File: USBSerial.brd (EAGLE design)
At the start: 45.8 x 26 mm, 28 parts, among them IC1 ATMEGA16U2, IC2 LD1117-33, J1 ISP, J2 USB, J5 DFU, J6 Serial, J8 Gnd, J9 VDD Select, Q1 16MHz

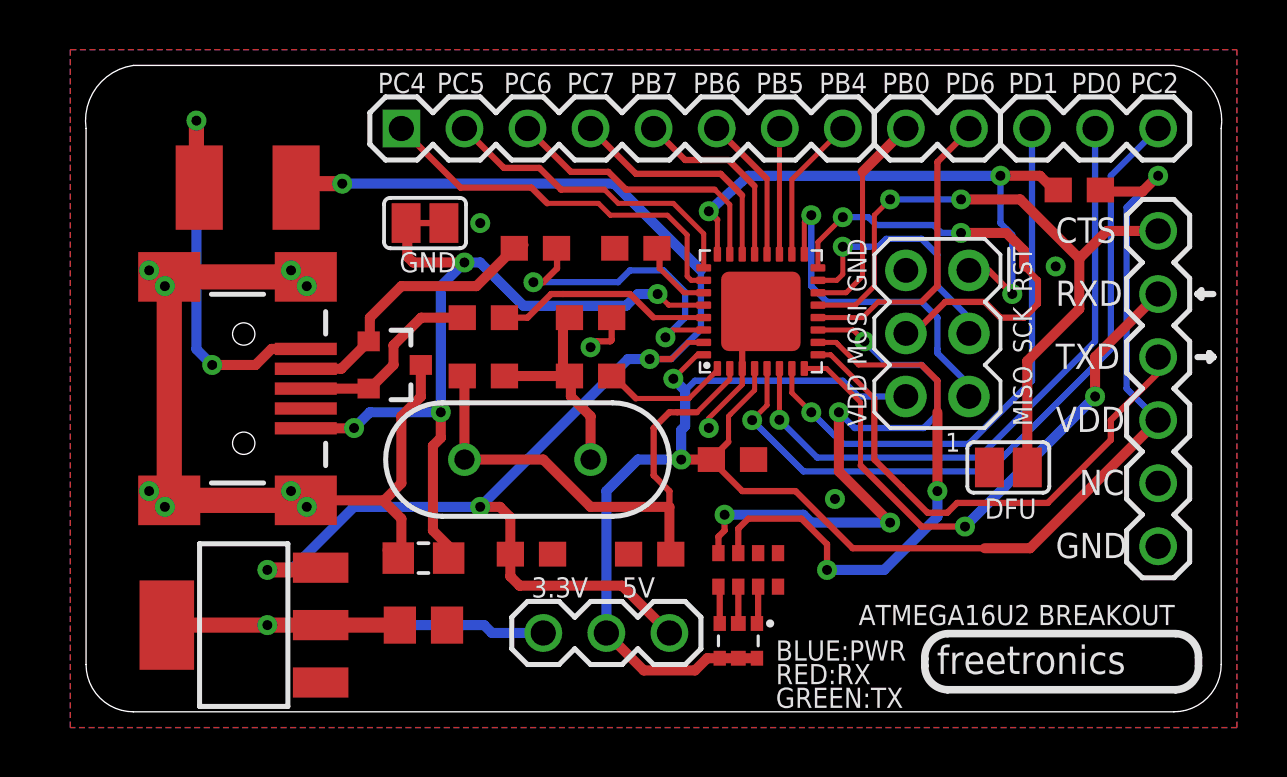
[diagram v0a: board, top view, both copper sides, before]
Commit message: Preparation for v1.0 release
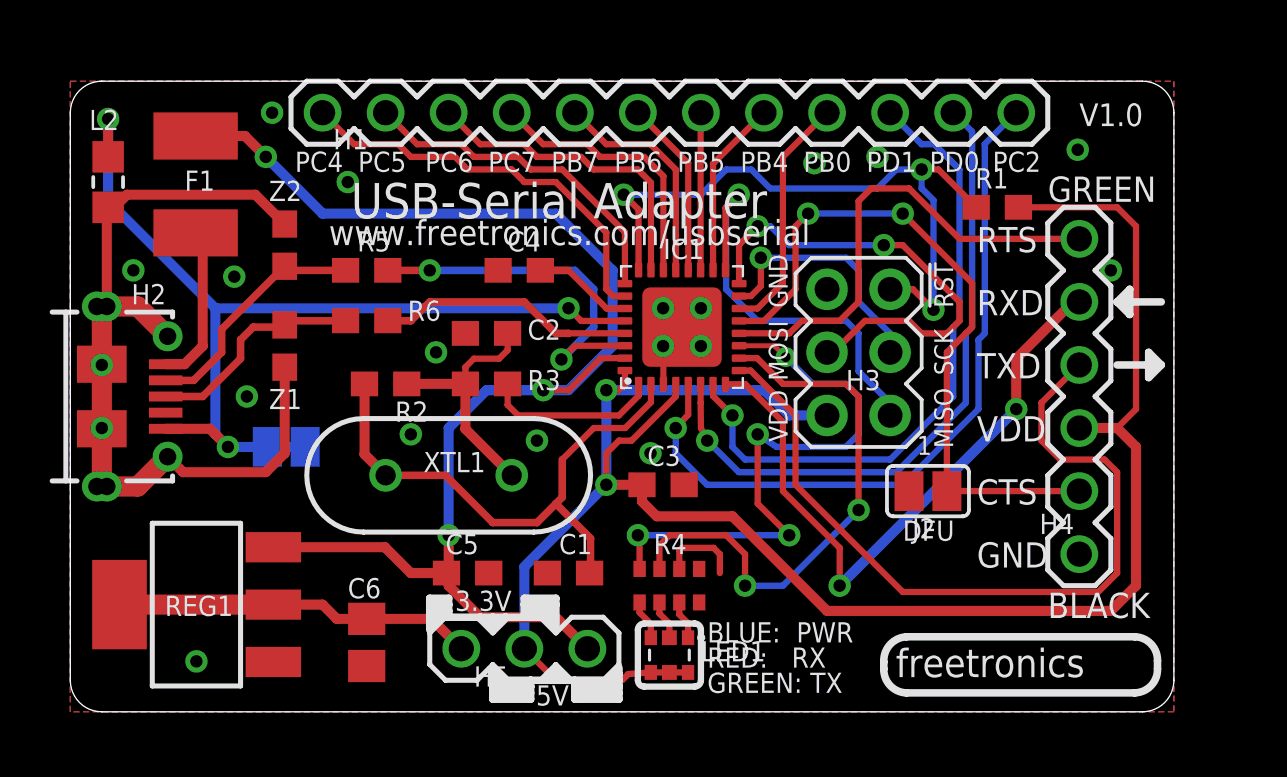
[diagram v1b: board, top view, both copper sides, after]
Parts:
- removed IC2: LD1117-33, freetronics-luke:SOT-223
- removed J3: (no value), freetronics-master-v1:1X02
- removed J4: (no value), freetronics-master-v1:1X08
- removed J5: DFU, freetronics-luke:SJ
- removed J6: Serial, freetronics-master-v1:1X06
- removed J7: (no value), freetronics-master-v1:1X03
- removed J8: Gnd, freetronics-luke:SJ
- removed J9: VDD Select, freetronics-luke:JUMPER_SPDT
- removed L1: Ferrite bead 0805, freetronics-master-v1:0805-LARGE
- removed Q1: 16MHz, freetronics-master-v1:HC49US
- added H1: M12PTH, freetronics-original:1X12
- added H2: USB-6PSMT, freetronics-jon:USB-MICROB-MB05PMXX
- added H3: ICSP, freetronics-luke:HEADER_2X3
- added H4: Serial, freetronics-master-v1:1X06
- added H5: VDD Select, freetronics-luke:JUMPER_SPDT
- added L2: 0805 INDUCTOR, freetronics-master-v1:0805-LARGE
- added REG1: LD1117-33 SOT-223, freetronics-luke:SOT-223
- added XTL1: 16MHz, freetronics-master-v1:HC49US
- added Z2: PGB1010603, freetronics:0603
- C1, C2: value 22p -> 22p 0603
- C3: value 100n -> 100n 0603
- C4: value 1uF -> 1uF 0603
- C5: value 10uF -> 100n 0603; device freetronics-jon:C0805 -> freetronics:0603
- C6: value 100n -> 10uF 10V ceramic 0805; device freetronics:0603 -> freetronics-jon:C0805
- F1: value 500mA PTC -> 500mA PTC 1812
- IC1: value ATMEGA16U2 -> ATMEGA16U2 QFN-32
- J1: value ISP -> Gnd; device freetronics-luke:HEADER_2X3 -> freetronics-jon:SJC
- J2: value USB -> DFU; device freetronics-luke:USB-MINIB-FT -> freetronics-luke:SJ
- R1: value 10k -> 10k 0603
- R2: value 1M -> 1M 0603
- R3: value 27R -> 27R 0603
- R5, R6: value 22R -> 22R 0603
- Z1: value PGB102ST23 -> PGB1010603; device freetronics-luke:SOT23-3 -> freetronics:0603
- moved J2 29.1 mm to (34.5, 8.89)
- moved J1 26.6 mm to (8.70, 10.7), flipped to the bottom, turned to 0 degrees
- moved C6 7.53 mm to (11.9, 2.79), turned to 270 degrees
- moved R5 6.85 mm to (11.9, 17.8)
- moved C4 4.78 mm to (18.1, 17.8)
- moved R6 4.70 mm to (11.9, 15.7)
- moved Z1 4.45 mm to (8.64, 14.7)
- moved C2 4.24 mm to (16.8, 15.2), turned to 0 degrees
- moved R3 4.20 mm to (16.8, 13.2)
- moved R2 3.95 mm to (12.7, 13.2)
- moved R1 3.38 mm to (37.3, 20.3)
- moved C1 3.36 mm to (20.1, 5.59)
- moved R4 3.24 mm to (24.1, 5.08)
- moved IC1 3.24 mm to (24.6, 15.5)
- moved C3 2.97 mm to (23.9, 9.14)
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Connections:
- removed net N$3: J2.SH1, J2.SH2, J2.SH3, J2.SH4, L1.1, Z1.3
- removed net PD6: IC1.12, J3.2
- new net N$8: H2.FIX1, H2.FIX2, H2.PIN1, H2.PIN2, H2.TAB1, H2.TAB2, L2.2, Z1.2, Z2.2
- new net RTS: H4.6, IC1.12
- net !RESET: now also H3.5; no longer J1.5
- net +3V3: now also C6.1, H5.1, REG1.2, REG1.4; no longer C5.1, IC2.2, IC2.4, J9.1
- net +5V: now also C5.1, H5.3, REG1.3; no longer C6.1, IC2.3, J9.3
- net CTS: now also H4.2, J2.2; no longer J5.2, J6.6
- net GND: now also H3.6, H4.1, J1.1, J2.1, REG1.1; no longer IC2.1, J1.6, J5.1, J6.1, J8.1
- net MISO: now also H3.1; no longer J1.1
- net MOSI: now also H3.4; no longer J1.4
- net N$1: now also H2.GND, J1.2, L2.1; no longer J2.GND, J8.2, L1.2
- net N$113: now also XTL1.2; no longer Q1.2
- net N$114: now also XTL1.1; no longer Q1.1
- net N$115: now also H2.VBUS; no longer J2.VBUS
- net N$16: now also H2.D+, Z1.1; no longer J2.D+, Z1.2
- net N$17: now also H2.D-, Z2.1; no longer J2.D-, Z1.1
- net PB0: now also H1.9; no longer J3.1
- net PB4: now also H1.8; no longer J4.8
- net PB5: now also H1.7; no longer J4.7
- net PB6: now also H1.6; no longer J4.6
- net PB7: now also H1.5; no longer J4.5
- net PC2: now also H1.12; no longer J7.1
- net PC4: now also H1.1; no longer J4.1
- net PC5: now also H1.2; no longer J4.2
- net PC6: now also H1.3; no longer J4.3
- net PC7: now also H1.4; no longer J4.4
- net PD0: now also H1.11; no longer J7.2
- net PD1: now also H1.10; no longer J7.3
- net RXD: now also H4.5; no longer J6.5
- net SCK: now also H3.3; no longer J1.3
- net TXD: now also H4.4; no longer J6.4
- net VDD: now also H3.2, H4.3, H5.2; no longer J1.2, J6.3, J9.2
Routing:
- net N$3: track 39.3 -> 0.00 mm, vias 8 -> 0
- net N$8: track 0.00 -> 34.0 mm, vias 0 -> 2
- net RTS: track 0.00 -> 19.3 mm
- net PD6: track 12.2 -> 0.00 mm
- net TXD: track 21.2 -> 32.2 mm
- net N$115: track 16.8 -> 6.47 mm, vias 2 -> 0
- net VDD: track 72.1 -> 82.1 mm, vias 3 -> 2
- net +3V3: track 21.3 -> 14.5 mm, vias 1 -> 0
- net N$1: track 32.9 -> 37.8 mm, vias 4 -> 3
- net !RESET: track 23.8 -> 27.4 mm
- net MISO: track 13.9 -> 17.2 mm
- net PD1: track 22.7 -> 26.0 mm
- net +5V: track 57.4 -> 54.4 mm, vias 4 -> 3
- net RXD: track 23.2 -> 26.0 mm
- net N$17: track 11.6 -> 9.76 mm
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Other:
- board size 45.8 x 26 mm -> 44.5 x 25.4 mm
- board text added: "ATMega16u2 16MHz"
- board text added: "BLACK"
- board text added: "BLUE: PWR"
- board text added: "GREEN"
- board text added: "GREEN: TX"
- board text added: "LED1"
- board text added: "RED: RX"
- board text added: "RTS"
- board text added: "USB-Serial Adapter"
- board text added: "V1.0"
- board text removed: "ATMEGA16U2 BREAKOUT"
- board text removed: "ATmega16U2 breakout board"
- board text removed: "BLK"
- board text removed: "BLUE:PWR"
- board text removed: "BRN"
- board text removed: "GREEN:TX"
- board text removed: "NC"
- board text removed: "ORN"
- board text removed: "PD6"
- board text removed: "RED"
- board text removed: "RED:RX"
- board text removed: "YEL"
